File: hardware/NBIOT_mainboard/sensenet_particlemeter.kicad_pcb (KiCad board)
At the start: 2 copper layers, 63.6 x 72.4 mm, 98 parts, among them J1 CONN_01X01, J11 CONN_01X01, J13 Conn_01x02_Female, J16 Conn_01x06_Female, J17 Conn_02x08_Odd_Even, J18 CONN_01X01, J19 CONN_01X01, J2 CONN_01X01, J20 Conn_02x04_Odd_Even, J21 CONN_01X01, J3 CONN_01X01, J4 CONN_01X01, J5 CONN_01X01, J6 CONN_01X01, J7 Conn_01x07_Female, J8 Conn_02x01, P1 SMA_mini, P2 SMA_mini, SW1 SW_DPST, SW3 SW_DPST, U1 NCP59152, U2 stm32f072, U3 QUECTEL_BC95, U4 SIM, U6 NCP59152, U7 M10578-A2, U8 ATECC508A

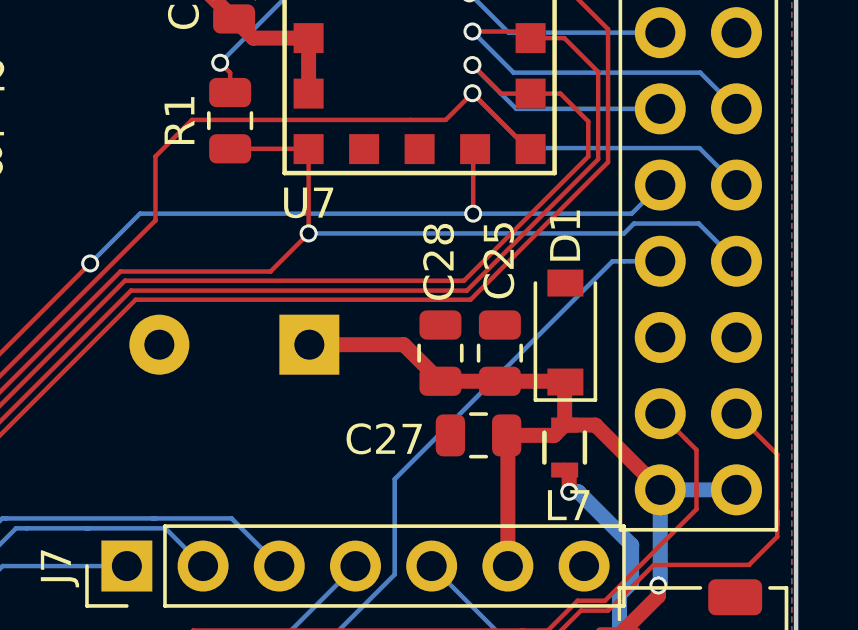
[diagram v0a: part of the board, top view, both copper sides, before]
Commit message: priprava FAB data
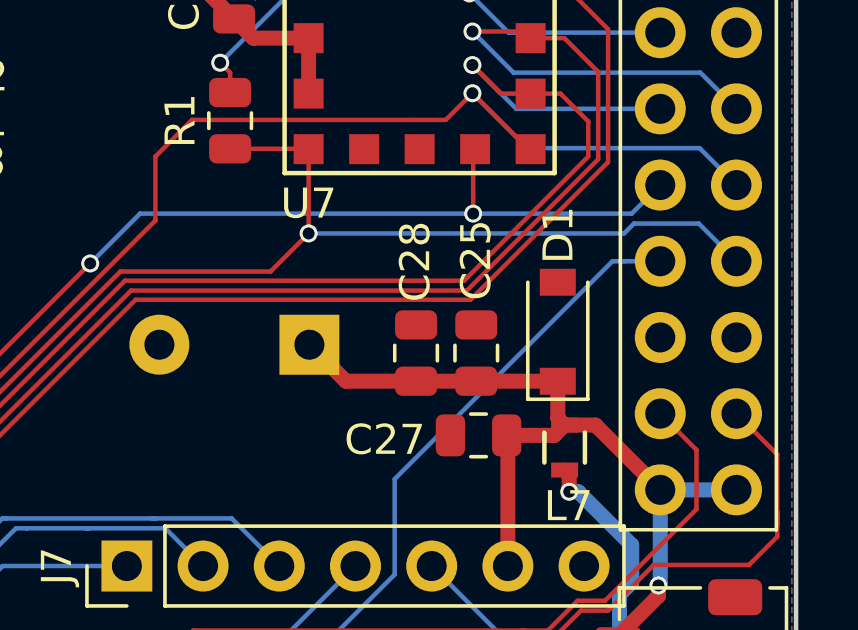
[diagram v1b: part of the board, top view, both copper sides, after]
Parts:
- D10: value GREEN -> LED GREEN
- moved C28 0.81 mm to (183.0, 77.7)
- moved C25 0.79 mm to (185.0, 77.7)
- moved D1 0.26 mm to (187.7, 77.0)
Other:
- net class Default: trace_width 0.4 -> 0.5
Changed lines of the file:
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@@
     (thickness 1.6)
     (drawings 92)
-    (tracks 1179)
+    (tracks 1181)
     (zones 0)
     (modules 98)
@@
   (layers
     (0 F.Cu signal)
-    (31 B.Cu signal)
+    (31 B.Cu signal hide)
     (32 B.Adhes user)
     (33 F.Adhes user)
@@
   )
   (setup
-    (last_trace_width 0.4)
+    (last_trace_width 0.5)
     (trace_clearance 0.15)
     (zone_clearance 0.2)
@@
       (drillshape 0)
       (scaleselection 1)
-      (outputdirectory "krivky/"))
+      (outputdirectory "FAB_outputs/machine/"))
   )
   (net 0 "")
@@
   (net_class Default "This is the default net class."
     (clearance 0.15)
-    (trace_width 0.4)
+    (trace_width 0.5)
     (via_dia 0.6)
     (via_drill 0.4)
@@
       (effects (font (size 1 1) (thickness 0.15)) (justify mirror))
     )
-    (fp_text value GREEN (at 0 1.75 180) (layer B.Fab)
+    (fp_text value "LED GREEN" (at 0 1.75 180) (layer B.Fab)
       (effects (font (size 1 1) (thickness 0.15)) (justify mirror))
     )
@@
   )
   (module Capacitor_SMD:C_0805_2012Metric (layer F.Cu)
-    (at 183.78932 77.68566 90)
+    (at 182.97652 77.68336 90)
     (descr "Capacitor SMD 0805 (2012 Metric), square (rectangular) end terminal, IPC_7351 nominal, (Body size source: https://docs.google.com/spreadsheets/d/1BsfQQcO9C6DZCsRaXUlFlo91Tg2WpOkGARC1WS5S8t0/edit?usp=sharing), generated with kicad-footprint-generator")
     (tags capacitor)
@@
   )
   (module Capacitor_SMD:C_0805_2012Metric (layer F.Cu)
-    (at 185.77052 77.68566 90)
+    (at 184.98312 77.68336 90)
     (descr "Capacitor SMD 0805 (2012 Metric), square (rectangular) end terminal, IPC_7351 nominal, (Body size source: https://docs.google.com/spreadsheets/d/1BsfQQcO9C6DZCsRaXUlFlo91Tg2WpOkGARC1WS5S8t0/edit?usp=sharing), generated with kicad-footprint-generator")
     (tags capacitor)
@@
   )
   (module Diode_SMD:D_SOD-123 (layer F.Cu)
-    (at 187.95492 76.99856 90)
+    (at 187.70092 76.97216 90)
     (descr SOD-123)
     (tags SOD-123)
@@
   (segment (start 191.05372 85.78216) (end 189.71452 87.12136) (width 0.5) (layer F.Cu) (net 3) (status 20))
   (segment (start 191.05372 85.43036) (end 191.05372 85.78216) (width 0.5) (layer F.Cu) (net 3))
-  (segment (start 183.78932 78.62316) (end 185.77052 78.62316) (width 0.5) (layer F.Cu) (net 3) (status 30))
   (segment (start 187.92952 78.62316) (end 187.95492 78.64856) (width 0.5) (layer F.Cu) (net 3) (status 30))
-  (segment (start 185.77052 78.62316) (end 187.92952 78.62316) (width 0.5) (layer F.Cu) (net 3) (status 30))
   (segment (start 187.58592 80.42656) (end 187.92952 80.08296) (width 0.5) (layer F.Cu) (net 3) (status 20))
   (segment (start 185.99682 80.42656) (end 187.58592 80.42656) (width 0.5) (layer F.Cu) (net 3) (status 10))
   (segment (start 187.92952 78.67396) (end 187.95492 78.64856) (width 0.5) (layer F.Cu) (net 3) (status 30))
-  (segment (start 187.92952 80.08296) (end 187.92952 78.67396) (width 0.5) (layer F.Cu) (net 3) (status 30))
-  (segment (start 182.57012 77.40396) (end 183.78932 78.62316) (width 0.5) (layer F.Cu) (net 3) (status 20))
-  (segment (start 179.42052 77.40396) (end 182.57012 77.40396) (width 0.5) (layer F.Cu) (net 3) (status 10))
   (segment (start 186.03722 80.46696) (end 185.99682 80.42656) (width 0.5) (layer F.Cu) (net 3) (status 30))
   (segment (start 186.03722 84.78266) (end 186.03722 80.46696) (width 0.5) (layer F.Cu) (net 3) (status 30))
@@
   (segment (start 187.92952 80.08296) (end 188.95752 80.08296) (width 0.5) (layer F.Cu) (net 3) (status 10))
   (segment (start 191.11722 82.24266) (end 193.65722 82.24266) (width 0.5) (layer B.Cu) (net 3) (status 30))
+  (segment (start 182.97652 78.62086) (end 184.98312 78.62086) (width 0.5) (layer F.Cu) (net 3) (status 30))
+  (segment (start 187.69962 78.62086) (end 187.70092 78.62216) (width 0.5) (layer F.Cu) (net 3) (status 30))
+  (segment (start 184.98312 78.62086) (end 187.69962 78.62086) (width 0.5) (layer F.Cu) (net 3) (status 30))
+  (segment (start 187.70092 79.85436) (end 187.92952 80.08296) (width 0.5) (layer F.Cu) (net 3) (status 30))
+  (segment (start 187.70092 78.62216) (end 187.70092 79.85436) (width 0.5) (layer F.Cu) (net 3) (status 30))
+  (segment (start 180.63742 78.62086) (end 179.42052 77.40396) (width 0.5) (layer F.Cu) (net 3) (status 20))
+  (segment (start 182.97652 78.62086) (end 180.63742 78.62086) (width 0.5) (layer F.Cu) (net 3) (status 10))
   (segment (start 191.1985 69.712754) (end 191.1985 69.469) (width 0.15) (layer F.Cu) (net 4) (status 30))
   (via (at 184.85612 68.08216) (size 0.6) (drill 0.4) (layers F.Cu B.Cu) (net 4))
